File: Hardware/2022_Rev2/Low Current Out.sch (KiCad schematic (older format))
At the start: 77 parts, among them Q10 FDC855N, Q11 IRLML2803TRPBF, Q3 FDC855N, Q4 IRLML2803TRPBF, Q6 IRLML2803TRPBF, Q7 IRLML2803TRPBF, Q8 FDC855N, Q9 FDC855N, U11 LT1910, U12 INA281, U13 INA281, U15 INA281, U16 INA281, U17 LT1910, U18 LT1910, U19 INA281, U20 LT1910, U21 LT1910, U22 LT1910, U23 INA281, U24 INA281, U25 INA281, U8 LT1910, U9 LT1910

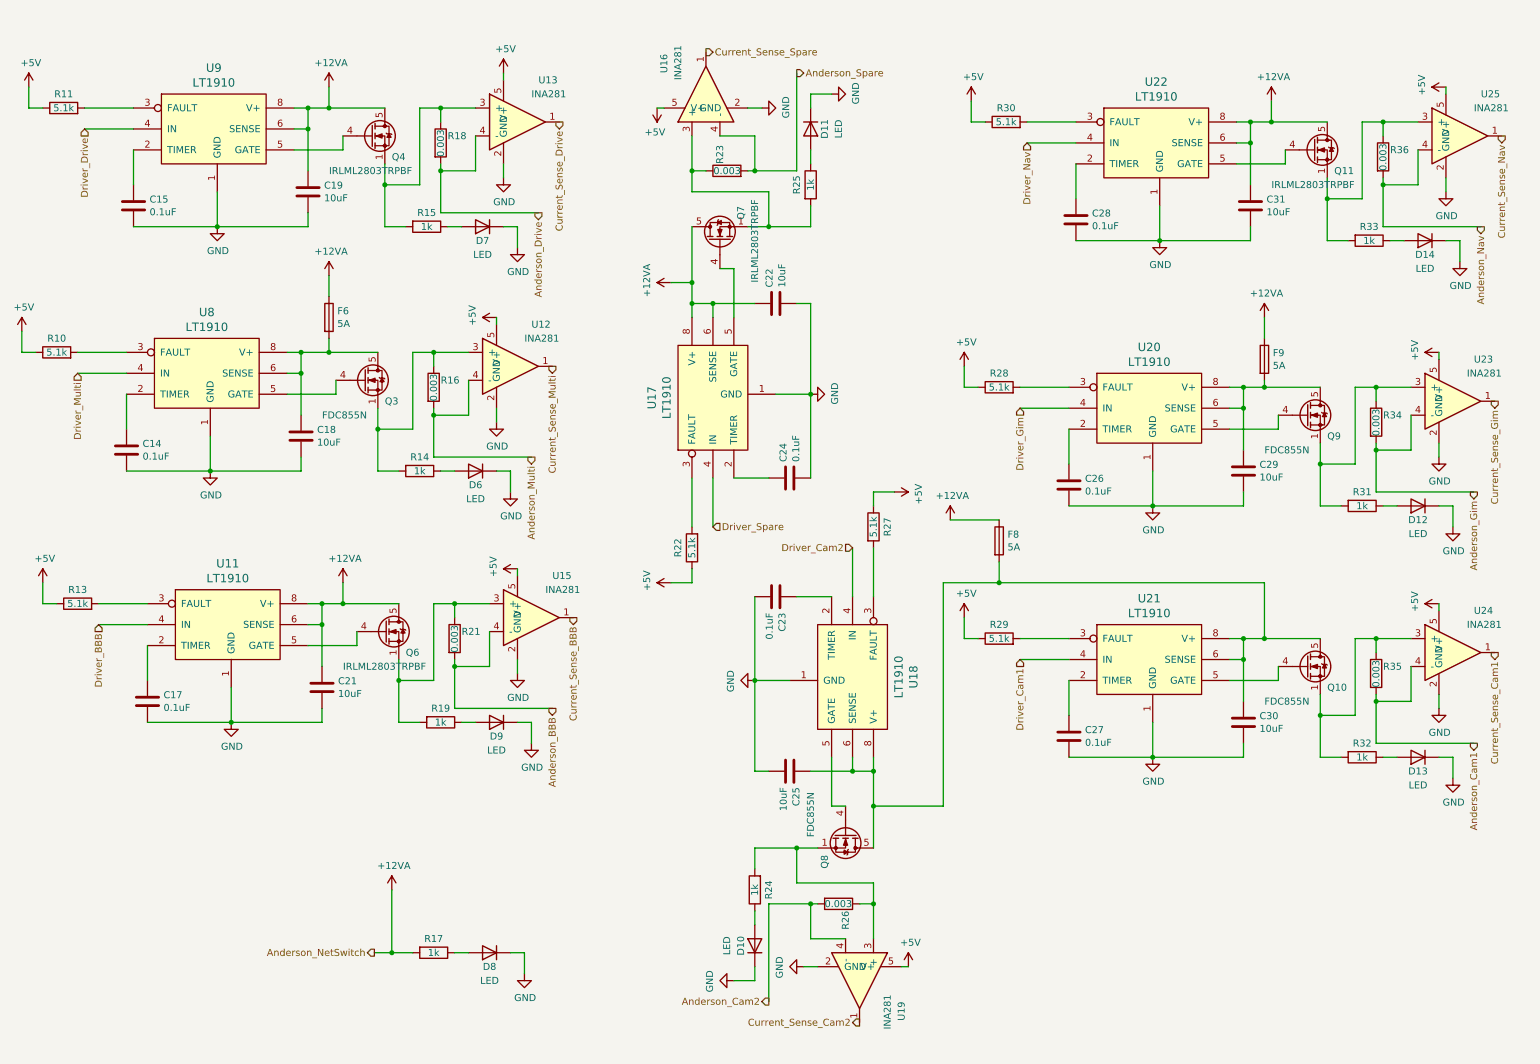
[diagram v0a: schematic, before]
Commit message: Gerbs are done
please review before you order this max
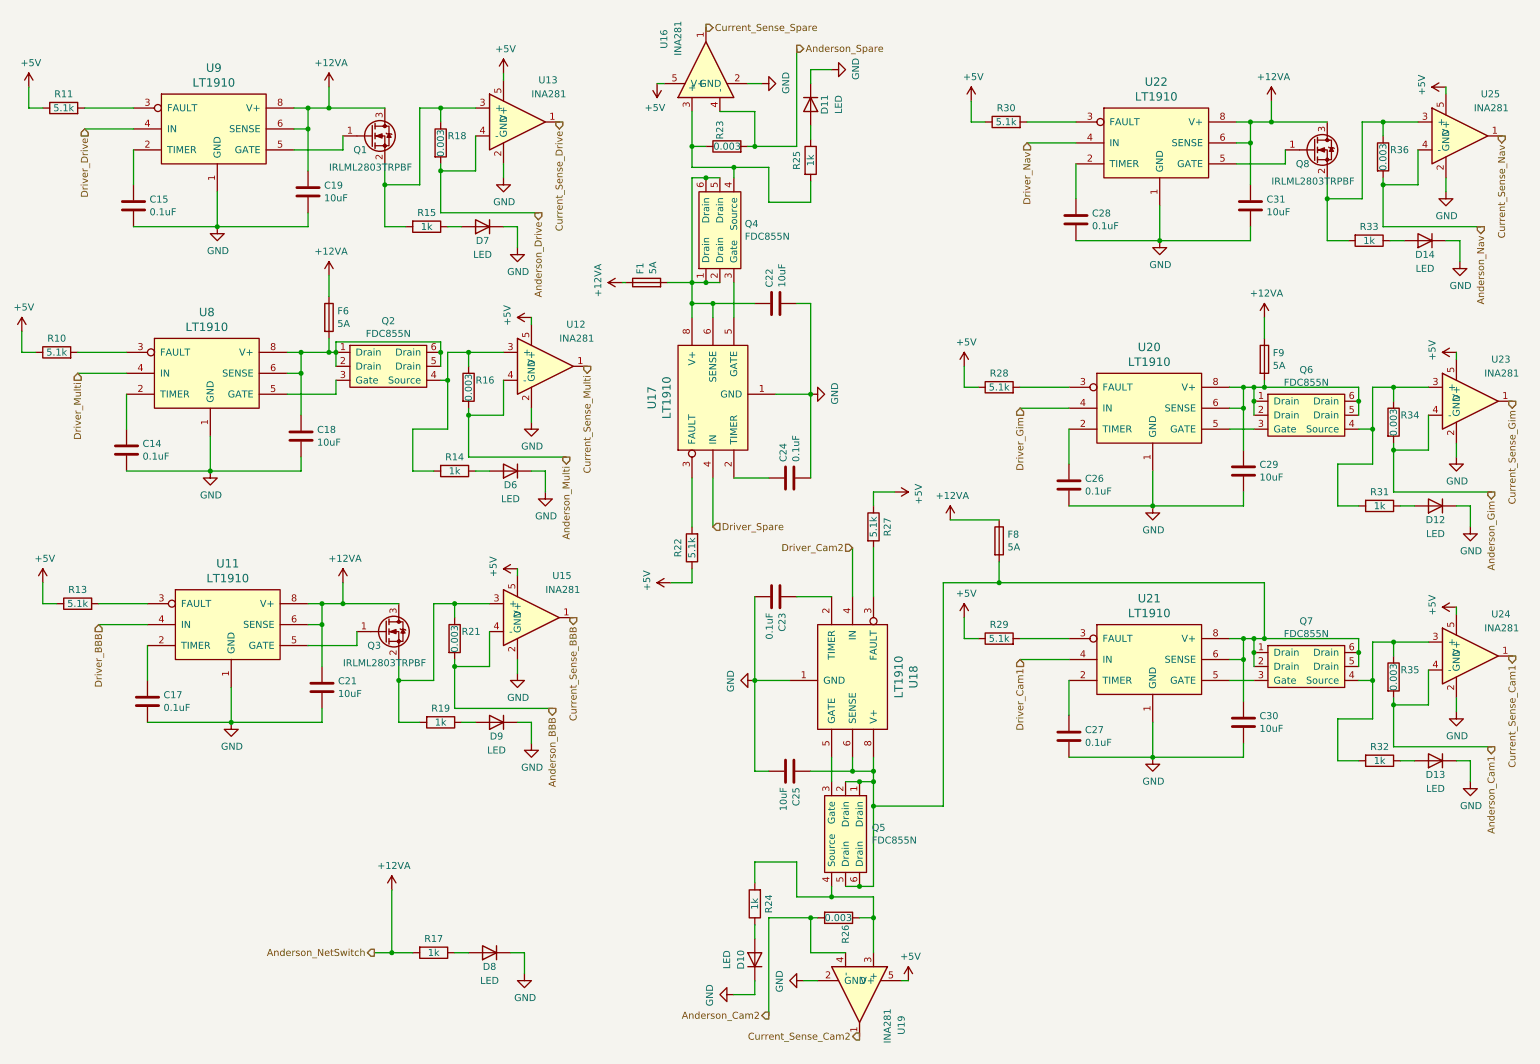
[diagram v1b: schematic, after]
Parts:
- removed Q10, Q3, Q8, Q9: FDC855N, Package_TO_SOT_SMD:SuperSOT-6, symbol Transistor_FET:BUK7M9R9-60EX
- removed Q11, Q4, Q6, Q7: IRLML2803TRPBF, Package_TO_SOT_SMD:SOT-23, symbol Transistor_FET:BUK7M9R9-60EX
- added F1: 5A, MRDT_Passives:ATC_Fuse_Block, symbol Device:Fuse
- added Q1, Q3, Q8: IRLML2803TRPBF, Package_TO_SOT_SMD:SOT-23, symbol Transistor_FET:IRLML0030
- added Q2, Q4, Q5, Q6, Q7: FDC855N, Package_TO_SOT_SMD:SuperSOT-6, symbol 12V_6A_Mosfet:FDC855N
- C14, C15, C17, C18, C19, C21, C22, C23, C24, C25, C26, C27, C28, C29, C30, C31: footprint Capacitor_SMD:C_0603_1608Metric_Pad1.08x0.95mm_HandSolder -> Capacitor_SMD:C_0603_1608Metric_Pad1.05x0.95mm_HandSolder
- R10, R11, R13, R14, R15, R17, R19, R22, R24, R25, R27, R28, R29, R30, R31, R32, R33: footprint Resistor_SMD:R_0603_1608Metric_Pad0.98x0.95mm_HandSolder -> Resistor_SMD:R_0603_1608Metric_Pad1.05x0.95mm_HandSolder
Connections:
- net +12VA: now also F1.1, Q1.3 (D), Q3.3 (D), Q8.3 (D); no longer C22.1, U17.6 (SENSE), U17.8 (V+)
- net at U11.5 (GATE): now also Q3.1 (G)
- net at R19.2, R21.1, U15.3 (+): now also Q3.2 (S)
- net at U8.5 (GATE): now also Q2.3 (Gate)
- net at C18.1, F6.2, U8.6 (SENSE)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: now also Q2.1 (Drain), Q2.2 (Drain), Q2.5 (Drain), Q2.6 (Drain)
- net at R14.2, R16.1, U12.3 (+): now also Q2.4 (Source)
- net at U9.5 (GATE): now also Q1.1 (G)
- net at R15.2, R18.1, U13.3 (+): now also Q1.2 (S)
- net at U22.5 (GATE): now also Q8.1 (G)
- net at R33.2, R36.1, U25.3 (+): now also Q8.2 (S)
- net at U20.5 (GATE): now also Q6.3 (Gate)
- net at C29.1, F9.2, U20.6 (SENSE)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: now also Q6.1 (Drain), Q6.2 (Drain), Q6.5 (Drain), Q6.6 (Drain)
- net at R31.2, R34.1, U23.3 (+): now also Q6.4 (Source)
- net at U21.5 (GATE): now also Q7.3 (Gate)
- net at C25.1, C30.1, F8.2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: now also Q5.1 (Drain), Q5.2 (Drain), Q5.5 (Drain), Q5.6 (Drain), Q7.1 (Drain), Q7.2 (Drain), Q7.5 (Drain), Q7.6 (Drain)
- net at R32.2, R35.1, U24.3 (+): now also Q7.4 (Source)
- net at U18.5 (GATE): now also Q5.3 (Gate)
- net at R24.2, R26.1, U19.3 (+): now also Q5.4 (Source)
- net at U17.5 (GATE): now also Q4.3 (Gate)
- net at R23.1, R25.2, U16.3 (+): now also Q4.4 (Source)
- new net: C22.1, F1.2, Q4.1 (Drain), Q4.2 (Drain), Q4.5 (Drain), Q4.6 (Drain), U17.6 (SENSE), U17.8 (V+)
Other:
- moved on the sheet: D10, D11, D12, D13, D6, R14, R16, R23, R24, R25, R26, R31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
